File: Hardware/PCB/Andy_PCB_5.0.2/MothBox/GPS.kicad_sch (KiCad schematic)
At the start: 15 parts, among them U10 Days, U11 Hours3, U12 MODE, U13 Hours1, U14 Hours2, U15 PCA9535PW, U16 PCA9535PW, U17 BH1750FVI-TR, U8 GPs 5 pin PM2.54-1*5, U9 PCA9535PW

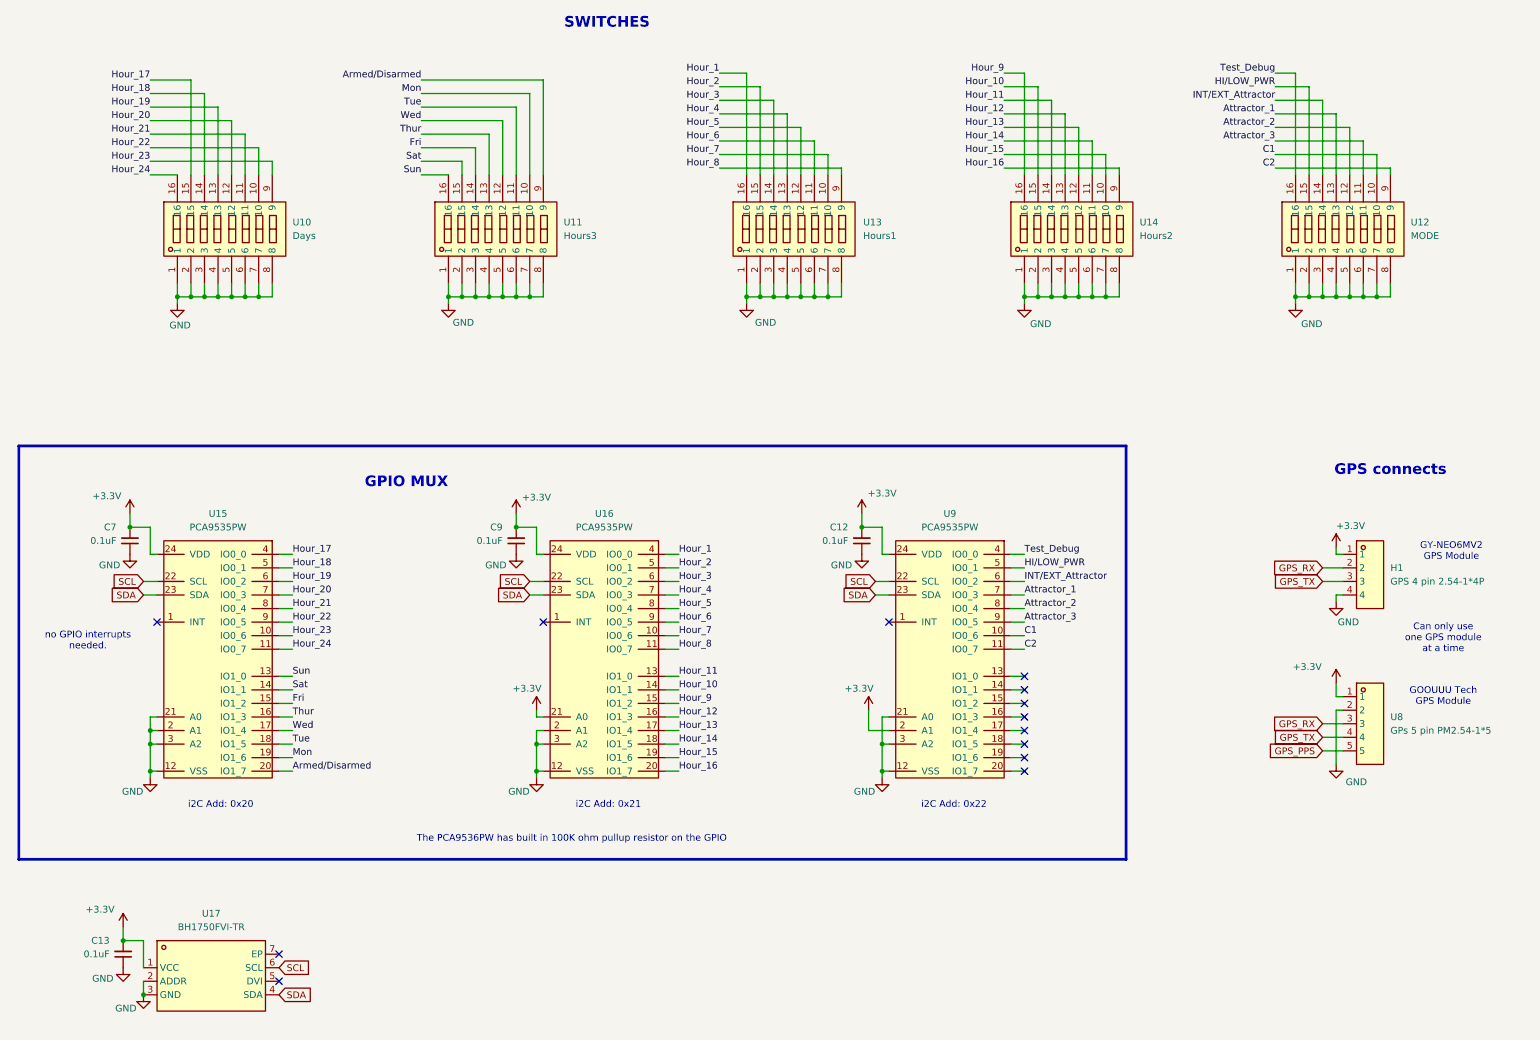
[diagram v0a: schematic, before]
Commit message: partial update on v5.0.2 modifications
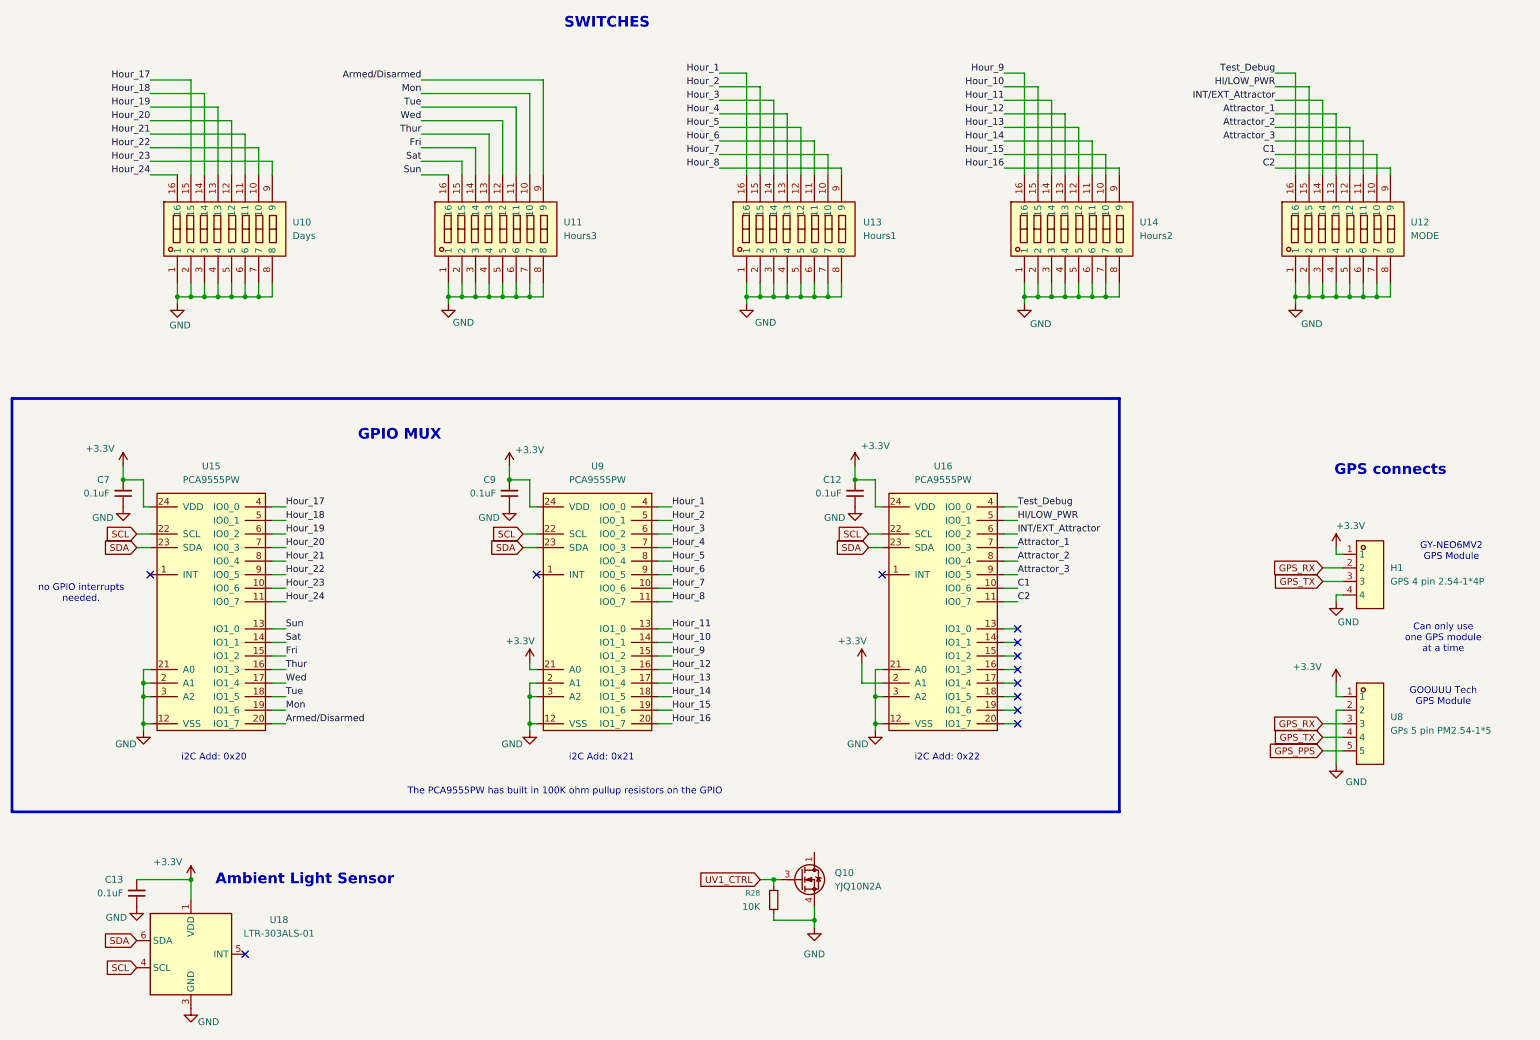
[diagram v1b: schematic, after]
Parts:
- removed U17: BH1750FVI-TR, easyeda2kicad:WSOF-6_L2.6-W1.6-P0.50-TL-EP, symbol easyeda2kicad:BH1750FVI-TR
- added Q10: YJQ10N2A, MothBox_footprints_Library:U-DFN2020-6_L2.0-W2.0-P0.65-BL, symbol MothBox_Symbol_Library:YJQ10N2A_1
- added R28: 10K, MothBox_footprints_Library:R_0603_1608Metric, symbol MothBox_Symbol_Library:R_Small
- added U18: LTR-303ALS-01, OptoDevice:Lite-On_LTR-303ALS-01, symbol Sensor_Optical:LTR-303ALS-01
- U15, U16, U9: value PCA9535PW -> PCA9555PW; LCSC_Part C255606 -> C42420607
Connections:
- net +3.3V: now also U16.2 (A1), U9.21 (A0), U18.1 (VDD); no longer U16.21 (A0), U9.2 (A1)
- net Attractor_1: now also U16.7 (IO0_3); no longer U9.7 (IO0_3)
- net Attractor_2: now also U16.8 (IO0_4); no longer U9.8 (IO0_4)
- net Attractor_3: now also U16.9 (IO0_5); no longer U9.9 (IO0_5)
- net C1: now also U16.10 (IO0_6); no longer U9.10 (IO0_6)
- net C2: now also U16.11 (IO0_7); no longer U9.11 (IO0_7)
- net GND: now also U16.21 (A0), U9.2 (A1), Q10.4 (S), Q10.7 (S), R28.2, U18.3 (GND); no longer U16.2 (A1), U9.21 (A0)
- net HI/LOW_PWR: now also U16.5 (IO0_1); no longer U9.5 (IO0_1)
- net Hour_1: now also U9.4 (IO0_0); no longer U16.4 (IO0_0)
- net Hour_10: now also U9.14 (IO1_1); no longer U16.14 (IO1_1)
- net Hour_11: now also U9.13 (IO1_0); no longer U16.13 (IO1_0)
- net Hour_12: now also U9.16 (IO1_3); no longer U16.16 (IO1_3)
- net Hour_13: now also U9.17 (IO1_4); no longer U16.17 (IO1_4)
- net Hour_14: now also U9.18 (IO1_5); no longer U16.18 (IO1_5)
- net Hour_15: now also U9.19 (IO1_6); no longer U16.19 (IO1_6)
- net Hour_16: now also U9.20 (IO1_7); no longer U16.20 (IO1_7)
- net Hour_2: now also U9.5 (IO0_1); no longer U16.5 (IO0_1)
- net Hour_3: now also U9.6 (IO0_2); no longer U16.6 (IO0_2)
- net Hour_4: now also U9.7 (IO0_3); no longer U16.7 (IO0_3)
- net Hour_5: now also U9.8 (IO0_4); no longer U16.8 (IO0_4)
- net Hour_6: now also U9.9 (IO0_5); no longer U16.9 (IO0_5)
- net Hour_7: now also U9.10 (IO0_6); no longer U16.10 (IO0_6)
- net Hour_8: now also U9.11 (IO0_7); no longer U16.11 (IO0_7)
- net Hour_9: now also U9.15 (IO1_2); no longer U16.15 (IO1_2)
- net INT/EXT_Attractor: now also U16.6 (IO0_2); no longer U9.6 (IO0_2)
- net SCL: now also U18.4 (SCL)
- net SDA: now also U18.6 (SDA)
- net Test_Debug: now also U16.4 (IO0_0); no longer U9.4 (IO0_0)
- new net: Q10.1 (D), Q10.2 (D), Q10.5 (D), Q10.6 (D), Q10.8 (D)
- new net UV1_CTRL: Q10.3 (G), R28.1
- no-connect marks 13 -> 12
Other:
- note added: "Ambient Light Sensor"
- note added: "The PCA9555PW has built in 100K ohm pullup resistors on the GPIO"
- note removed: "The PCA9536PW has built in 100K ohm pullup resistor on the GPIO"
- moved on the sheet: C12, C13, C7, C9, U15
